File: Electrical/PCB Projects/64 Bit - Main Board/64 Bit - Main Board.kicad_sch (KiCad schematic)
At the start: 0 parts

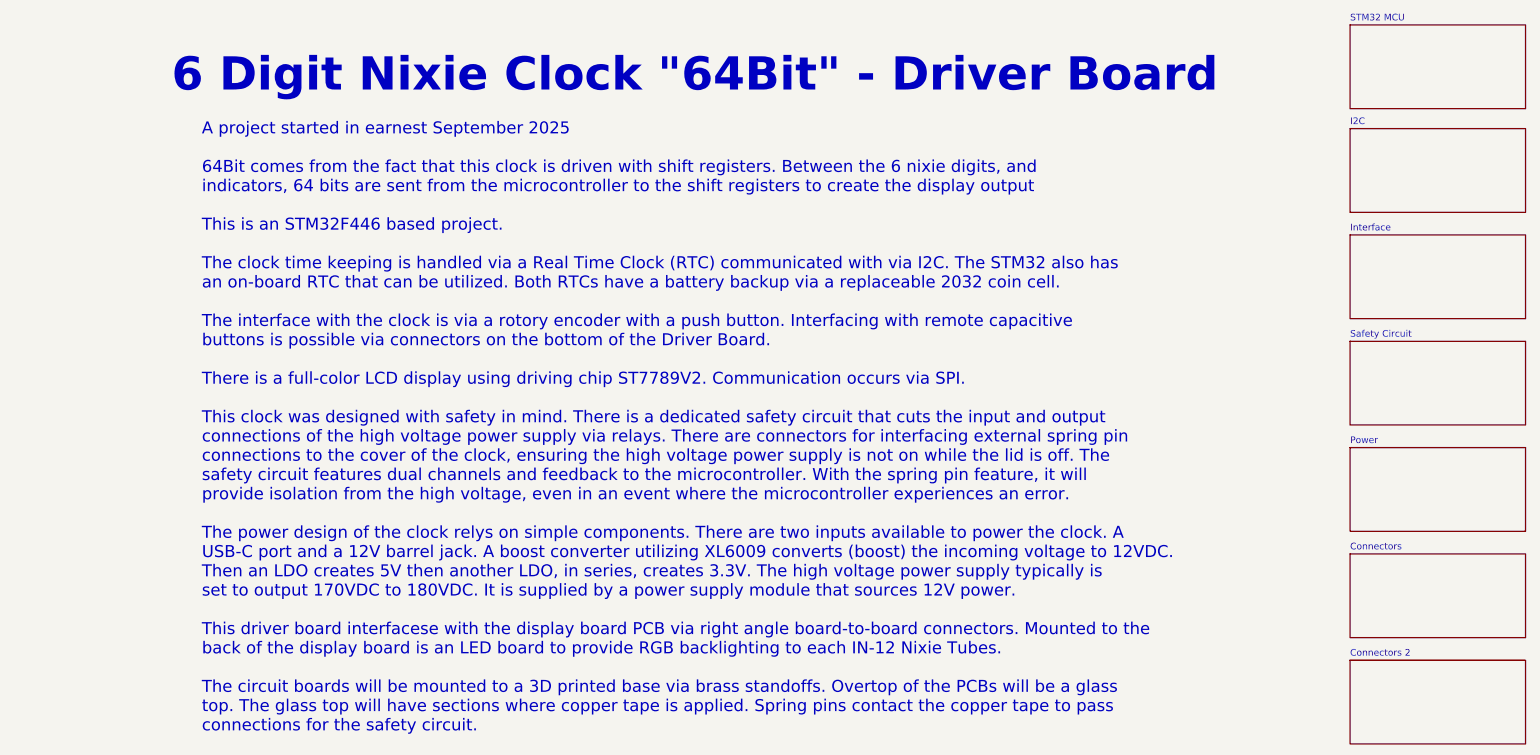
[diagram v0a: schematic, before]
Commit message: simple text update in sch proj, git test
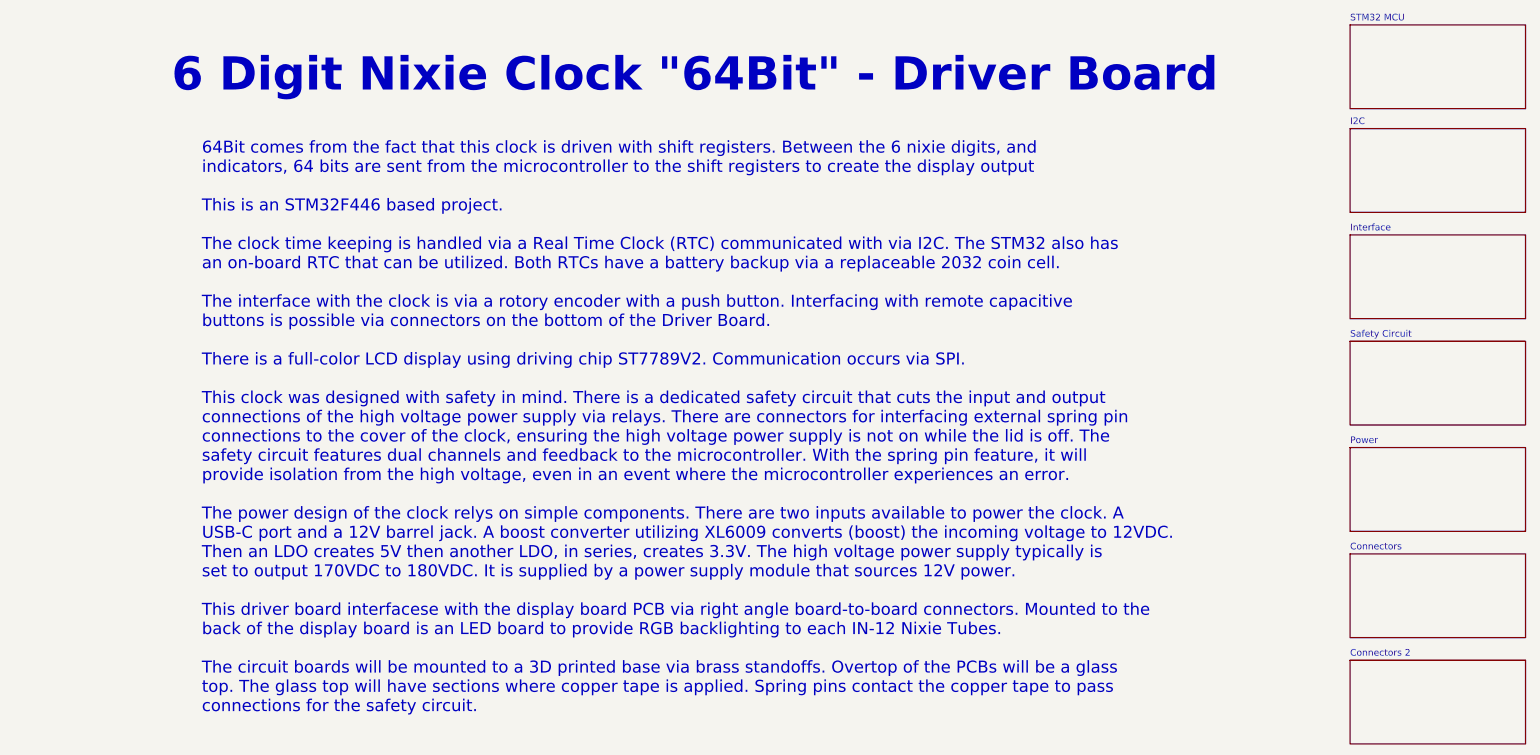
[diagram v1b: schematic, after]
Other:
- note added: "64Bit comes from the fact that this clock is driven with shift registers. Between the 6 nixie digits, and indicators, 64 bits are sent from the microcontroller to the shift registers to create the display output This is an STM32F446 based project. The clock time keeping is handled via a Real Time Clock (RTC) communicated with via I2C. The STM32 also has an on-board RTC that can be utilized. Both 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"
- note removed: "A project started in earnest September 2025 64Bit comes from the fact that this clock is driven with shift registers. Between the 6 nixie digits, and indicators, 64 bits are sent from the microcontroller to the shift registers to create the display output This is an STM32F446 based project. The clock time keeping is handled via a Real Time Clock (RTC) communicated with via I2C. The STM32 also has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"
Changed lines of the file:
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@@
 		(company "Kadin Whiting")
 	)
-	(text "A project started in earnest September 2025\n\n64Bit comes from the fact that this clock is driven with shift registers. Between the 6 nixie digits, and \nindicators, 64 bits are sent from the microcontroller to the shift registers to create the display output\n\nThis is an STM32F446 based project. \n\nThe clock time keeping is handled via a Real Time Clock (RTC) communicated with via I2C. The STM32 also has \nan on-board RTC that can be utilized. Both RTCs have a battery backup via a replaceable 2032 coin cell.\n\nThe interface with the clock is via a rotory encoder with a push button. Interfacing with remote capacitive\nbuttons is possible via connectors on the bottom of the Driver Board.\n\nThere is a full-color LCD display using driving chip ST7789V2. Communication occurs via SPI.\n\nThis clock was designed with safety in mind. There is a dedicated safety circuit that cuts the input and output \nconnections of the high voltage power supply via relays. There are connectors for interfacing external spring pin \nconnections to the cover of the clock, ensuring the high voltage power supply is not on while the lid is off. The \nsafety circuit features dual channels and feedback to the microcontroller. With the spring pin feature, it will \nprovide isolation from the high voltage, even in an event where the microcontroller experiences an error.\n\nThe power design of the clock relys on simple components. There are two inputs available to power the clock. A \nUSB-C port and a 12V barrel jack. A boost converter utilizing XL6009 converts (boost) the incoming voltage to 12VDC. \nThen an LDO creates 5V then another LDO, in series, creates 3.3V. The high voltage power supply typically is \nset to output 170VDC to 180VDC. It is supplied by a power supply module that sources 12V power.\n\nThis driver board interfacese with the display board PCB via right angle board-to-board connectors. Mounted to the \nback of the display board is an LED board to provide RGB backlighting to each IN-12 Nixie Tubes.\n\nThe circuit boards will be mounted to a 3D printed base via brass standoffs. Overtop of the PCBs will be a glass \ntop. The glass top will have sections where copper tape is applied. Spring pins contact the copper tape to pass \nconnections for the safety circuit. "
+	(text "64Bit comes from the fact that this clock is driven with shift registers. Between the 6 nixie digits, and \nindicators, 64 bits are sent from the microcontroller to the shift registers to create the display output\n\nThis is an STM32F446 based project. \n\nThe clock time keeping is handled via a Real Time Clock (RTC) communicated with via I2C. The STM32 also has \nan on-board RTC that can be utilized. Both RTCs have a battery backup via a replaceable 2032 coin cell.\n\nThe interface with the clock is via a rotory encoder with a push button. Interfacing with remote capacitive\nbuttons is possible via connectors on the bottom of the Driver Board.\n\nThere is a full-color LCD display using driving chip ST7789V2. Communication occurs via SPI.\n\nThis clock was designed with safety in mind. There is a dedicated safety circuit that cuts the input and output \nconnections of the high voltage power supply via relays. There are connectors for interfacing external spring pin \nconnections to the cover of the clock, ensuring the high voltage power supply is not on while the lid is off. The \nsafety circuit features dual channels and feedback to the microcontroller. With the spring pin feature, it will \nprovide isolation from the high voltage, even in an event where the microcontroller experiences an error.\n\nThe power design of the clock relys on simple components. There are two inputs available to power the clock. A \nUSB-C port and a 12V barrel jack. A boost converter utilizing XL6009 converts (boost) the incoming voltage to 12VDC. \nThen an LDO creates 5V then another LDO, in series, creates 3.3V. The high voltage power supply typically is \nset to output 170VDC to 180VDC. It is supplied by a power supply module that sources 12V power.\n\nThis driver board interfacese with the display board PCB via right angle board-to-board connectors. Mounted to the \nback of the display board is an LED board to provide RGB backlighting to each IN-12 Nixie Tubes.\n\nThe circuit boards will be mounted to a 3D printed base via brass standoffs. Overtop of the PCBs will be a glass \ntop. The glass top will have sections where copper tape is applied. Spring pins contact the copper tape to pass \nconnections for the safety circuit. "
 		(exclude_from_sim no)
 		(at 28.194 92.71 0)
